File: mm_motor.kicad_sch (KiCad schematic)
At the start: 3 parts, among them J2 Conn_01x06_Pin, M1 N20_encoder

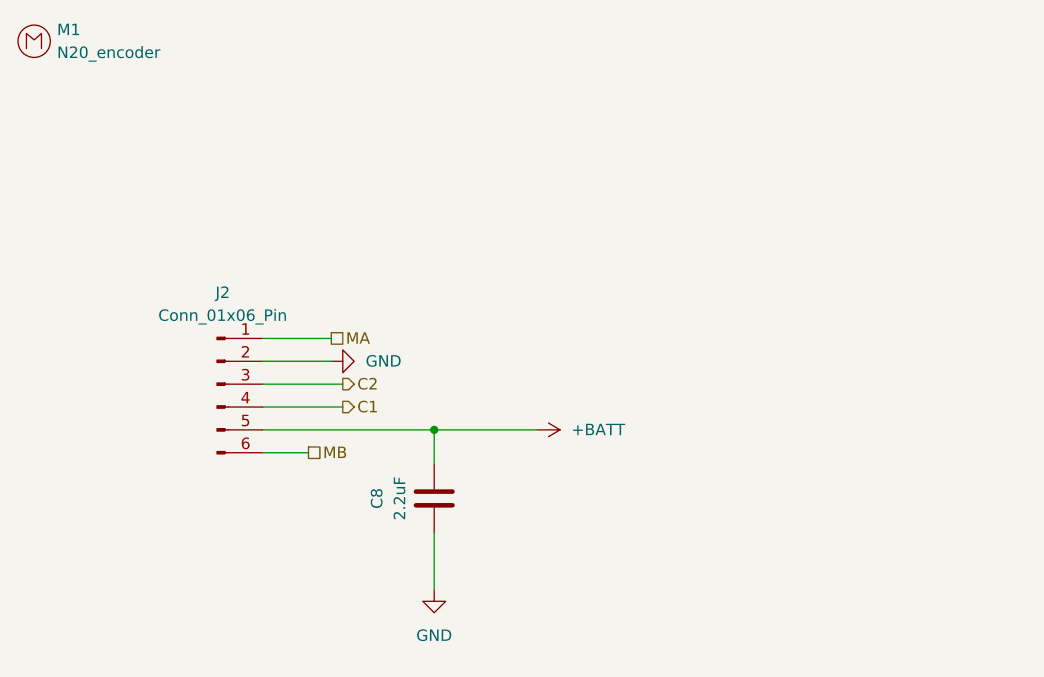
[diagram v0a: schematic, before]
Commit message: version 3
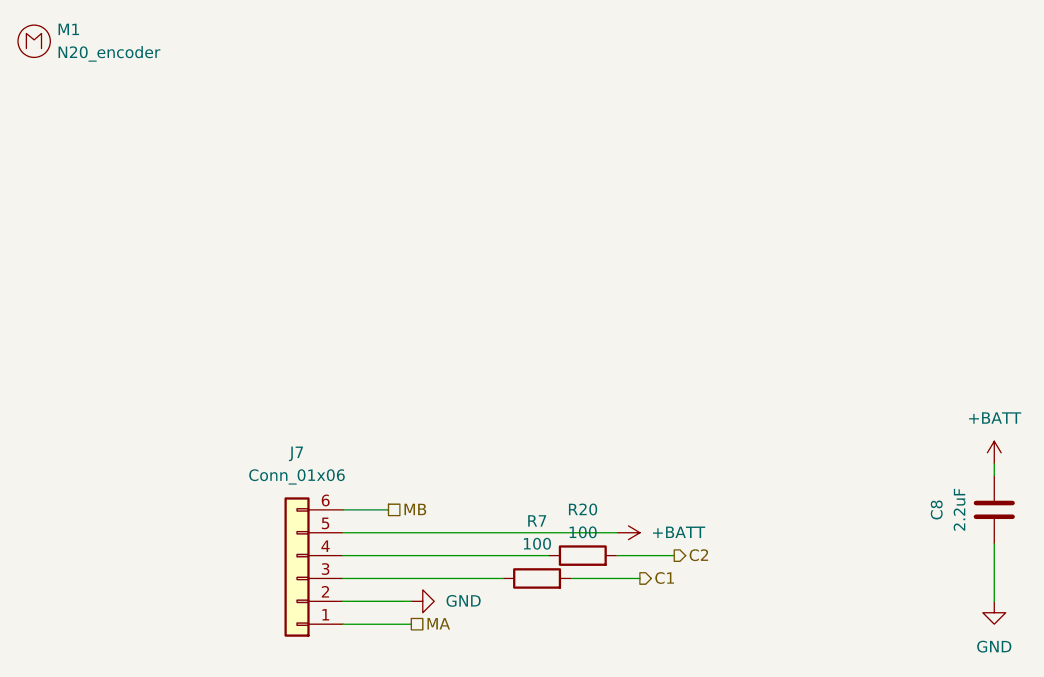
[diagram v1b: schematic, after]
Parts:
- removed J2: Conn_01x06_Pin, symbol Connector:Conn_01x06_Pin
- added J7: Conn_01x06, Connector_PinHeader_2.54mm:PinHeader_1x06_P2.54mm_Vertical, symbol Connector_Generic:Conn_01x06
- added R20, R7: 100, Resistor_SMD:R_0603_1608Metric, symbol Device:R
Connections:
- net +BATT: now also J7.5 (Pin_5)
- net C1: now also R7.2
- net C2: now also R20.2
- net GND: now also J7.2 (Pin_2)
- net MA: now also J7.1 (Pin_1)
- net MB: now also J7.6 (Pin_6)
- new net: J7.3 (Pin_3), R7.1
- new net: J7.4 (Pin_4), R20.1
